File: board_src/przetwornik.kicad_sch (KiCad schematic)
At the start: 3 parts, among them IC5 MCP3202-CI_MS, J23 Conn_01x04, J4 Conn_01x04

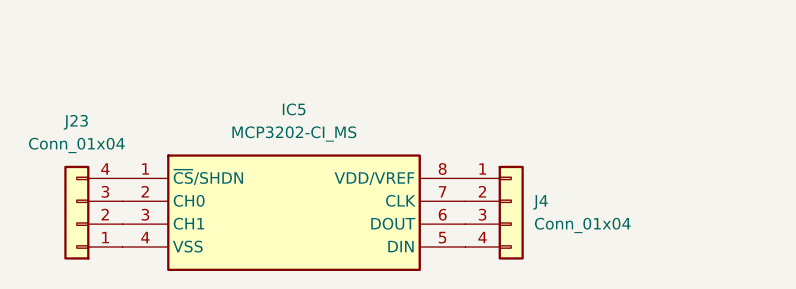
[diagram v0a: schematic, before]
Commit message: wersja uzupelnione footprinty
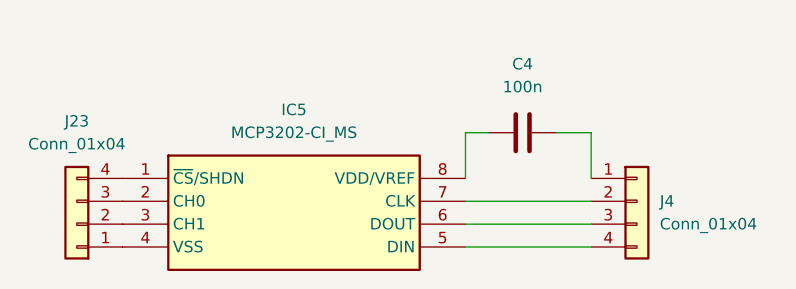
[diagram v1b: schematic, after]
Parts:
- added C4: 100n, Capacitor_SMD:C_1808_4520Metric, symbol Device:C
- J23, J4: footprint (none) -> Connector_PinHeader_2.54mm:PinHeader_1x04_P2.54mm_Vertical
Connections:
- net at J4.1 (Pin_1): now also C4.2; no longer IC5.8 (VDD/VREF)
- new net: C4.1, IC5.8 (VDD/VREF)
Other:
- moved on the sheet: J4
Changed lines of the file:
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@@
 	(generator_version "9.0")
 	(paper "A4")
+	(wire
+		(pts
+			(xy 129.54 86.36) (xy 115.57 86.36)
+		)
+		(stroke
+			(width 0)
+			(type default)
+		)
+	)
+	(wire
+		(pts
+			(xy 129.54 88.9) (xy 115.57 88.9)
+		)
+		(stroke
+			(width 0)
+			(type default)
+		)
+	)
+	(wire
+		(pts
+			(xy 115.57 76.2) (xy 118.11 76.2)
+		)
+		(stroke
+			(width 0)
+			(type default)
+		)
+	)
+	(wire
+		(pts
+			(xy 115.57 81.28) (xy 115.57 76.2)
+		)
+		(stroke
+			(width 0)
+			(type default)
+		)
+	)
+	(wire
+		(pts
+			(xy 129.54 83.82) (xy 115.57 83.82)
+		)
+		(stroke
+			(width 0)
+			(type default)
+		)
+	)
+	(wire
+		(pts
+			(xy 125.73 76.2) (xy 129.54 76.2)
+		)
+		(stroke
+			(width 0)
+			(type default)
+		)
+	)
+	(wire
+		(pts
+			(xy 129.54 76.2) (xy 129.54 81.28)
+		)
+		(stroke
+			(width 0)
+			(type default)
+		)
+	)
 	(symbol
 		(lib_id "Connector_Generic:Conn_01x04")
-		(at 120.65 83.82 0)
+		(at 134.62 83.82 0)
 		(unit 1)
 		(exclude_from_sim no)
@@
 		(fields_autoplaced yes)
 		(property "Reference" "J4"
-			(at 123.19 83.8199 0)
+			(at 137.16 83.8199 0)
 			(effects
 				(font
@@
 		)
 		(property "Value" "Conn_01x04"
-			(at 123.19 86.3599 0)
+			(at 137.16 86.3599 0)
 			(effects
 				(font
@@
 			)
 		)
-		(property "Footprint" ""
-			(at 120.65 83.82 0)
+		(property "Footprint" "Connector_PinHeader_2.54mm:PinHeader_1x04_P2.54mm_Vertical"
+			(at 134.62 83.82 0)
 			(effects
 				(font
@@
 		)
 		(property "Datasheet" "~"
-			(at 120.65 83.82 0)
+			(at 134.62 83.82 0)
 			(effects
 				(font
@@
 		)
 		(property "Description" "Generic connector, single row, 01x04, script generated (kicad-library-utils/schlib/autogen/connector/)"
-			(at 120.65 83.82 0)
+			(at 134.62 83.82 0)
 			(effects
 				(font
@@
 				(path "/772e9f49-cfcf-4cf6-843d-0684684f2d4b/72381f9f-0261-4c9d-a878-5b854177e01f"
 					(reference "J4")
+					(unit 1)
+				)
+			)
+		)
+	)
+	(symbol
+		(lib_id "Device:C")
+		(at 121.92 76.2 90)
+		(unit 1)
+		(exclude_from_sim no)
+		(in_bom yes)
+		(on_board yes)
+		(dnp no)
+		(fields_autoplaced yes)
+		(property "Reference" "C4"
+			(at 121.92 68.58 90)
+			(effects
+				(font
+					(size 1.27 1.27)
+				)
+			)
+		)
+		(property "Value" "100n"
+			(at 121.92 71.12 90)
+			(effects
+				(font
+					(size 1.27 1.27)
+				)
+			)
+		)
+		(property "Footprint" "Capacitor_SMD:C_1808_4520Metric"
+			(at 125.73 75.2348 0)
+			(effects
+				(font
+					(size 1.27 1.27)
+				)
+				(hide yes)
+			)
+		)
+		(property "Datasheet" "~"
+			(at 121.92 76.2 0)
+			(effects
+				(font
+					(size 1.27 1.27)
+				)
+				(hide yes)
+			)
+		)
+		(property "Description" "Unpolarized capacitor"
+			(at 121.92 76.2 0)
+			(effects
+				(font
+					(size 1.27 1.27)
+				)
+				(hide yes)
+			)
+		)
+		(pin "2"
+		)
+		(pin "1"
+		)
+		(instances
+			(project ""
+				(path "/772e9f49-cfcf-4cf6-843d-0684684f2d4b/72381f9f-0261-4c9d-a878-5b854177e01f"
+					(reference "C4")
 					(unit 1)
 				)
@@
 			)
 		)
-		(property "Footprint" ""
+		(property "Footprint" "Connector_PinHeader_2.54mm:PinHeader_1x04_P2.54mm_Vertical"
 			(at 72.39 86.36 0)
 			(effects

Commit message: wersja z FT232RN
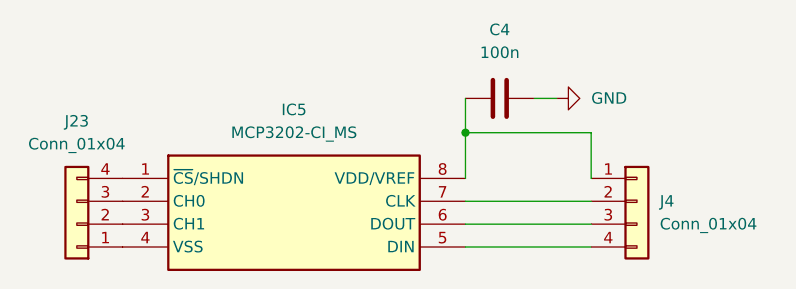
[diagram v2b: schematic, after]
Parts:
- C4: footprint Capacitor_SMD:C_1808_4520Metric -> Capacitor_SMD:C_1206_3216Metric_Pad1.33x1.80mm_HandSolder
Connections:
- net at J4.1 (Pin_1): now also C4.1, IC5.8 (VDD/VREF); no longer C4.2
- new net GND: C4.2
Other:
- moved on the sheet: C4
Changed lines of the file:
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@@
 	(generator_version "9.0")
 	(paper "A4")
+	(junction
+		(at 115.57 76.2)
+		(diameter 0)
+		(color 0 0 0 0)
+	)
 	(wire
 		(pts
@@
 	(wire
 		(pts
+			(xy 123.19 72.39) (xy 125.73 72.39)
+		)
+		(stroke
+			(width 0)
+			(type default)
+		)
+	)
+	(wire
+		(pts
 			(xy 129.54 88.9) (xy 115.57 88.9)
 		)
@@
 	(wire
 		(pts
-			(xy 115.57 76.2) (xy 118.11 76.2)
+			(xy 115.57 76.2) (xy 129.54 76.2)
+		)
+		(stroke
+			(width 0)
+			(type default)
+		)
+	)
+	(wire
+		(pts
+			(xy 115.57 72.39) (xy 115.57 76.2)
 		)
 		(stroke
@@
 		(pts
 			(xy 129.54 83.82) (xy 115.57 83.82)
-		)
-		(stroke
-			(width 0)
-			(type default)
-		)
-	)
-	(wire
-		(pts
-			(xy 125.73 76.2) (xy 129.54 76.2)
 		)
 		(stroke
@@
 	)
 	(symbol
+		(lib_id "power:GND")
+		(at 125.73 72.39 90)
+		(unit 1)
+		(exclude_from_sim no)
+		(in_bom yes)
+		(on_board yes)
+		(dnp no)
+		(fields_autoplaced yes)
+		(property "Reference" "#PWR041"
+			(at 132.08 72.39 0)
+			(effects
+				(font
+					(size 1.27 1.27)
+				)
+				(hide yes)
+			)
+		)
+		(property "Value" "GND"
+			(at 129.54 72.3899 90)
+			(effects
+				(font
+					(size 1.27 1.27)
+				)
+				(justify right)
+			)
+		)
+		(property "Footprint" ""
+			(at 125.73 72.39 0)
+			(effects
+				(font
+					(size 1.27 1.27)
+				)
+				(hide yes)
+			)
+		)
+		(property "Datasheet" ""
+			(at 125.73 72.39 0)
+			(effects
+				(font
+					(size 1.27 1.27)
+				)
+				(hide yes)
+			)
+		)
+		(property "Description" "Power symbol creates a global label with name \"GND\" , ground"
+			(at 125.73 72.39 0)
+			(effects
+				(font
+					(size 1.27 1.27)
+				)
+				(hide yes)
+			)
+		)
+		(pin "1"
+		)
+		(instances
+			(project ""
+				(path "/772e9f49-cfcf-4cf6-843d-0684684f2d4b/72381f9f-0261-4c9d-a878-5b854177e01f"
+					(reference "#PWR041")
+					(unit 1)
+				)
+			)
+		)
+	)
+	(symbol
 		(lib_id "Device:C")
-		(at 121.92 76.2 90)
+		(at 119.38 72.39 90)
 		(unit 1)
 		(exclude_from_sim no)
@@
 		(fields_autoplaced yes)
 		(property "Reference" "C4"
-			(at 121.92 68.58 90)
+			(at 119.38 64.77 90)
 			(effects
 				(font
@@
 		)
 		(property "Value" "100n"
-			(at 121.92 71.12 90)
-			(effects
-				(font
-					(size 1.27 1.27)
-				)
-			)
-		)
-		(property "Footprint" "Capacitor_SMD:C_1808_4520Metric"
-			(at 125.73 75.2348 0)
+			(at 119.38 67.31 90)
+			(effects
+				(font
+					(size 1.27 1.27)
+				)
+			)
+		)
+		(property "Footprint" "Capacitor_SMD:C_1206_3216Metric_Pad1.33x1.80mm_HandSolder"
+			(at 123.19 71.4248 0)
 			(effects
 				(font
@@
 		)
 		(property "Datasheet" "~"
-			(at 121.92 76.2 0)
+			(at 119.38 72.39 0)
 			(effects
 				(font
@@
 		)
 		(property "Description" "Unpolarized capacitor"
-			(at 121.92 76.2 0)
-			(effects
-				(font
+			(at 119.38 72.39 0)
+			(effects
+				(font
